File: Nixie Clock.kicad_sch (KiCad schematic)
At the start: 6 parts, among them J1 USB_C_Receptacle_USB2.0, U1 ESP32-S2-WROVER

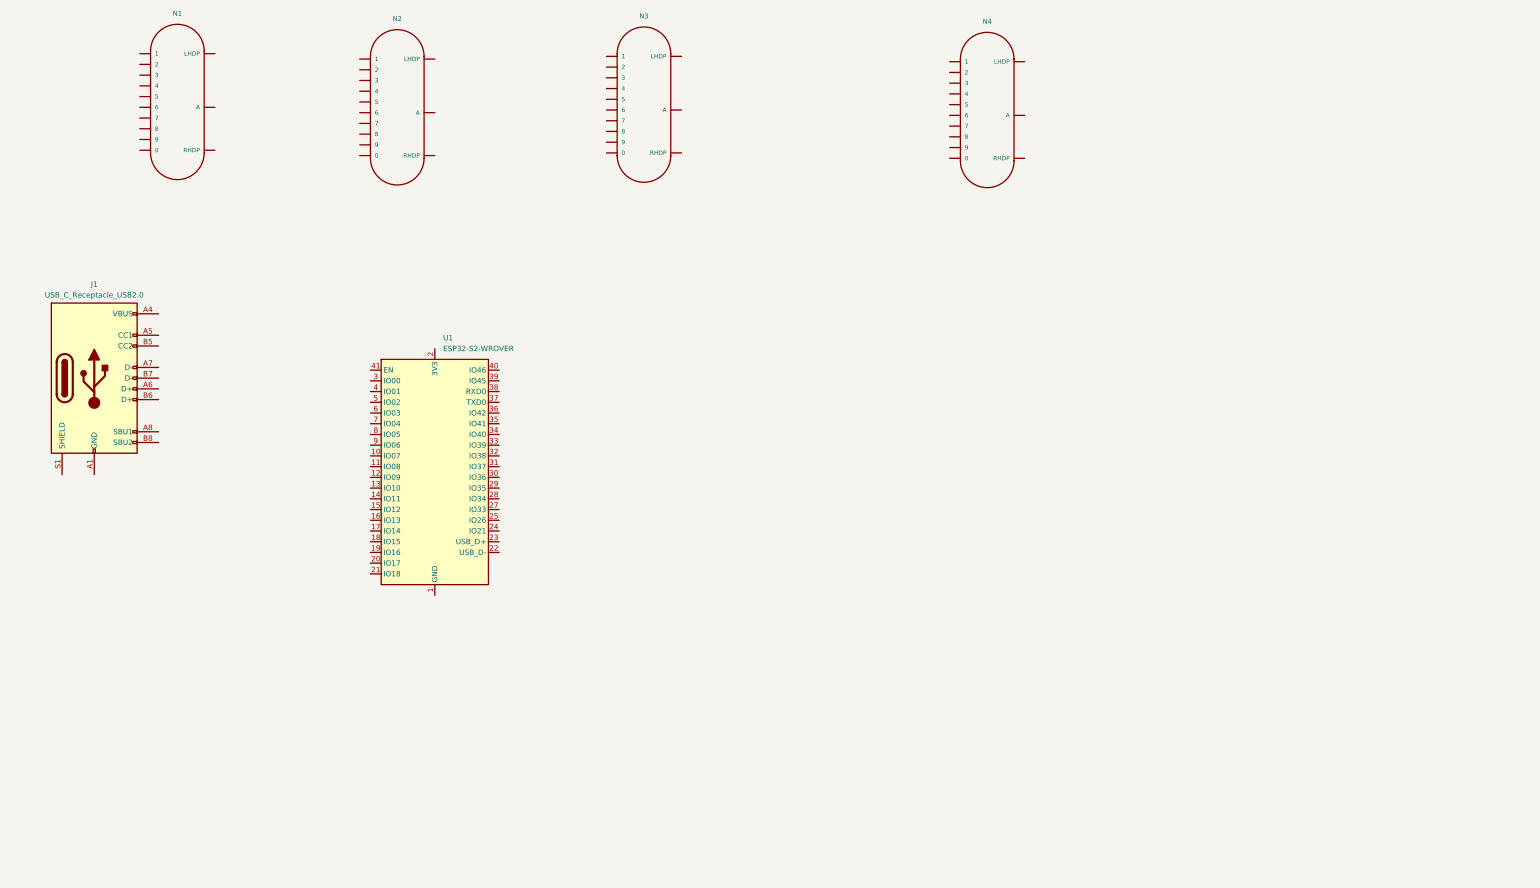
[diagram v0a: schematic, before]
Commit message: Finalized Bottom Plate with Gerbers
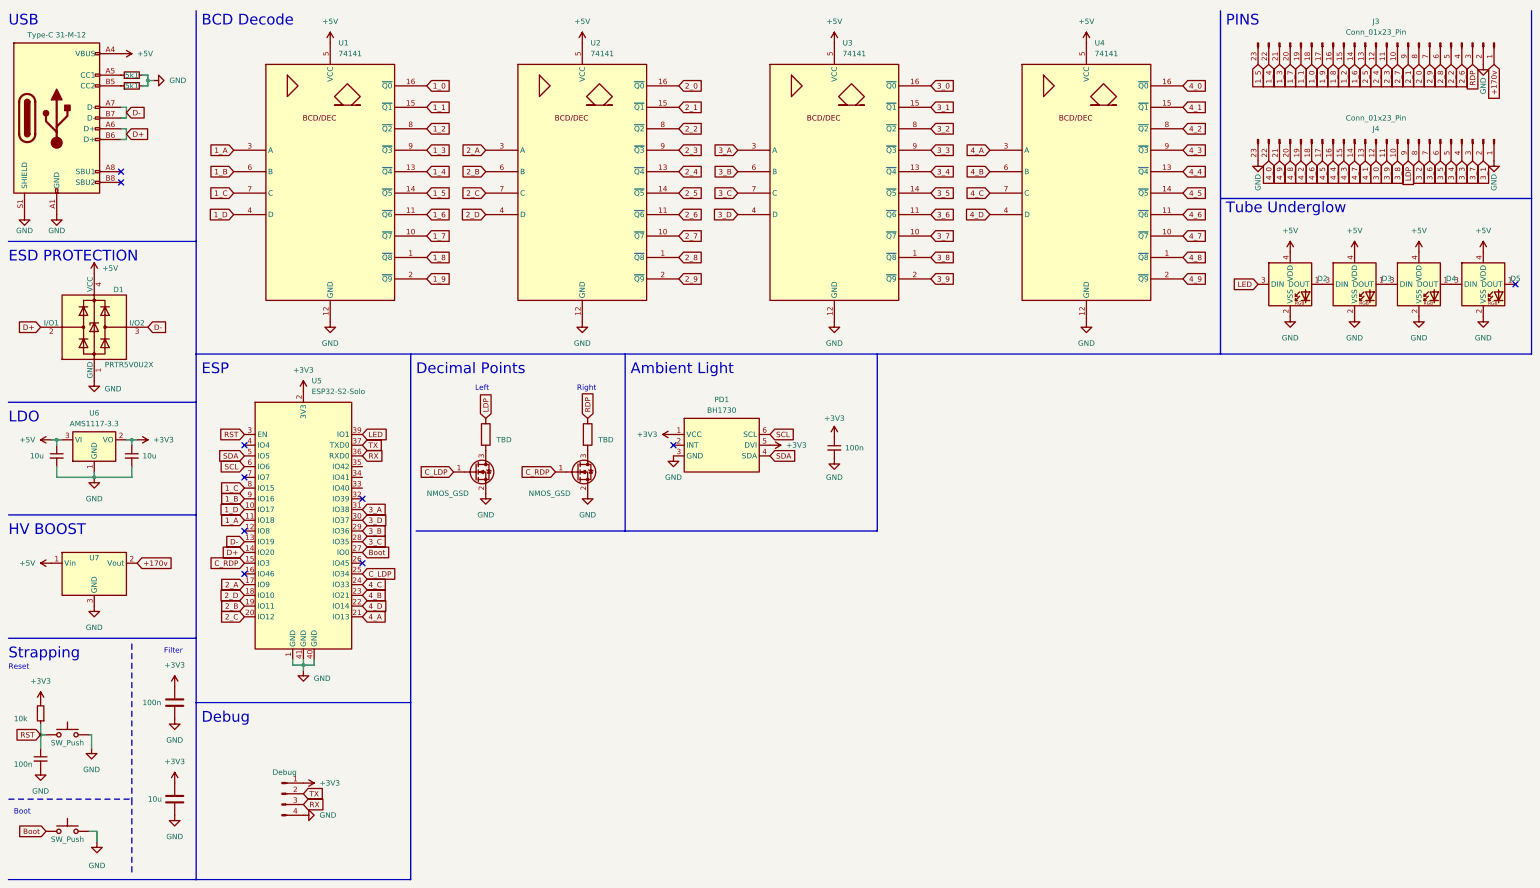
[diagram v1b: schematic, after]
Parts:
- removed N1, N2, N3, N4: IN-16, nixies-us:nixies-us-IN-16, symbol nixies-us:IN-16
- removed U1: ESP32-S2-WROVER, RF_Module:ESP32-S3-WROOM-1, symbol RF_Module:ESP32-S2-WROVER
- added C1, C2: 10u, Capacitor_SMD:C_0603_1608Metric, symbol Device:C_Small
- added C3: 10u, Capacitor_SMD:C_0603_1608Metric, symbol Device:C
- added C4: 100n, Capacitor_SMD:C_0402_1005Metric, symbol Device:C
- added C5, C6: 100n, Capacitor_SMD:C_0402_1005Metric, symbol Device:C_Small
- added D1: PRTR5V0U2X, Package_TO_SOT_SMD:SOT-143, symbol Power_Protection:PRTR5V0U2X
- added D2, D3, D4, D5: ~, LED_SMD:LED_WS2812B-2020_PLCC4_2.0x2.0mm, symbol WorldSemi_LED:WS2812B-2020
- added J2: Debug, Connector_PinHeader_2.54mm:PinHeader_1x04_P2.54mm_Vertical, symbol Connector:Conn_01x04_Pin
- added J3, J4: Conn_01x23_Pin, Connector_PinSocket_2.54mm:PinSocket_1x23_P2.54mm_Vertical, symbol Connector:Conn_01x23_Pin
- added PD1: BH1730, Sensor_Ambient:WSOF6, symbol BH1730:BH1730
- added Q1, Q2: NMOS_GSD, Package_TO_SOT_SMD:SOT-23, symbol Device:Q_NMOS_GSD
- added R1, R2: 5k1, Resistor_SMD:R_0402_1005Metric, symbol Device:R_Small
- added R3: 10k, Resistor_SMD:R_0402_1005Metric, symbol Device:R_Small
- added R4, R5: TBD, Resistor_SMD:R_0603_1608Metric_Pad0.98x0.95mm_HandSolder, symbol Device:R
- added RST1, SW2: SW_Push, Button_Switch_SMD:SW_SPST_SKQG_WithStem, symbol Switch:SW_Push
- added U1, U2, U3, U4: 74141, Package_DIP:DIP-16_W7.62mm, symbol 74xx_IEEE:74141
- added U5: ESP32-S2-Solo, RF_Module:ESP32-S3-WROOM-1, symbol ESP:ESP32-S2-Solo
- added U6: AMS1117-3.3, Package_TO_SOT_SMD:SOT-223-3_TabPin2, symbol Regulator_Linear:AMS1117-3.3
- added U7: ~, omnixie:8200HV, symbol omnixie:8200HV
- J1: value USB_C_Receptacle_USB2.0 -> Type-C 31-M-12
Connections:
- net GND: now reaches J1.A1 (GND), J1.A12 (GND), J1.B1 (GND), J1.B12 (GND)
- net GND: now also J1.S1 (SHIELD), C1.2, C2.2, C3.2, C4.2, C5.2, C6.2, D1.1 (GND), D2.2 (VSS), D3.2 (VSS), D4.2 (VSS), D5.2 (VSS), J2.4 (Pin_4), J3.2 (Pin_2), J4.1 (Pin_1), J4.23 (Pin_23), PD1.3 (GND), Q1.2 (S), Q2.2 (S), R1.2, R2.2, RST1.2, SW2.2, U1.12 (GND), U2.12 (GND), U3.12 (GND), U4.12 (GND), U5.1 (GND), U5.40 (GND), U5.41 (GND), U6.1 (GND), U7.3 (GND)
- net +5V: now reaches J1.A4 (VBUS), J1.A9 (VBUS), J1.B4 (VBUS), J1.B9 (VBUS)
- net +5V: now also C1.1, D1.4 (VCC), D2.4 (VDD), D3.4 (VDD), D4.4 (VDD), D5.4 (VDD), U1.5 (VCC), U2.5 (VCC), U3.5 (VCC), U4.5 (VCC), U6.3 (VI), U7.1 (Vin)
- net at J1.A5 (CC1): now also R1.1
- net D+: now reaches J1.A6 (D+)
- net D+: now also J1.B6 (D+), D1.2 (I/O1), U5.14 (IO20)
- net D-: now reaches J1.A7 (D-)
- net D-: now also J1.B7 (D-), D1.3 (I/O2), U5.13 (IO19)
- net at J1.B5 (CC2): now also R2.1
- new net: D4.1 (DOUT), D5.3 (DIN)
- new net: D3.1 (DOUT), D4.3 (DIN)
- new net: Q1.3 (D), R4.2
- new net: Q2.3 (D), R5.2
- new net: D2.1 (DOUT), D3.3 (DIN)
- new net +170v: J3.1 (Pin_1), U7.2 (Vout)
- new net +3V3: C2.1, C3.1, C4.1, C6.1, J2.1 (Pin_1), PD1.1 (VCC), PD1.5 (DVI), R3.2, U5.2 (3V3), U6.2 (VO)
- new net 1_0: J3.18 (Pin_18), U1.16 (~{Q0})
- new net 1_1: J3.19 (Pin_19), U1.15 (~{Q1})
- new net 1_2: J3.15 (Pin_15), U1.8 (~{Q2})
- new net 1_3: J3.21 (Pin_21), U1.9 (~{Q3})
- new net 1_4: J3.22 (Pin_22), U1.13 (~{Q4})
- new net 1_5: J3.23 (Pin_23), U1.14 (~{Q5})
- new net 1_6: J3.14 (Pin_14), U1.11 (~{Q6})
- new net 1_7: J3.20 (Pin_20), U1.10 (~{Q7})
- new net 1_8: J3.16 (Pin_16), U1.1 (~{Q8})
- new net 1_9: J3.17 (Pin_17), U1.2 (~{Q9})
- new net 1_A: U1.3 (A), U5.11 (IO18)
- new net 1_B: U1.6 (B), U5.9 (IO16)
- new net 1_C: U1.7 (C), U5.8 (IO15)
- new net 1_D: U1.4 (D), U5.10 (IO17)
- new net 2_0: J3.8 (Pin_8), U2.16 (~{Q0})
- new net 2_1: J3.9 (Pin_9), U2.15 (~{Q1})
- new net 2_2: J3.5 (Pin_5), U2.8 (~{Q2})
- new net 2_3: J3.11 (Pin_11), U2.9 (~{Q3})
- new net 2_4: J3.12 (Pin_12), U2.13 (~{Q4})
- new net 2_5: J3.13 (Pin_13), U2.14 (~{Q5})
- new net 2_6: J3.4 (Pin_4), U2.11 (~{Q6})
- new net 2_7: J3.10 (Pin_10), U2.10 (~{Q7})
- new net 2_8: J3.6 (Pin_6), U2.1 (~{Q8})
- new net 2_9: J3.7 (Pin_7), U2.2 (~{Q9})
- new net 2_A: U2.3 (A), U5.17 (IO9)
- new net 2_B: U2.6 (B), U5.19 (IO11)
- new net 2_C: U2.7 (C), U5.20 (IO12)
- new net 2_D: U2.4 (D), U5.18 (IO10)
- new net 3_0: J4.12 (Pin_12), U3.16 (~{Q0})
- new net 3_1: J4.2 (Pin_2), U3.15 (~{Q1})
- new net 3_2: J4.8 (Pin_8), U3.8 (~{Q2})
- new net 3_3: J4.4 (Pin_4), U3.9 (~{Q3})
- new net 3_4: J4.5 (Pin_5), U3.13 (~{Q4})
- new net 3_5: J4.6 (Pin_6), U3.14 (~{Q5})
- new net 3_6: J4.7 (Pin_7), U3.11 (~{Q6})
- new net 3_7: J4.3 (Pin_3), U3.10 (~{Q7})
- new net 3_8: J4.10 (Pin_10), U3.1 (~{Q8})
- new net 3_9: J4.11 (Pin_11), U3.2 (~{Q9})
- new net 3_A: U3.3 (A), U5.31 (IO38)
- new net 3_B: U3.6 (B), U5.29 (IO36)
- new net 3_C: U3.7 (C), U5.28 (IO35)
- new net 3_D: U3.4 (D), U5.30 (IO37)
- new net 4_0: J4.22 (Pin_22), U4.16 (~{Q0})
- new net 4_1: J4.13 (Pin_13), U4.15 (~{Q1})
- new net 4_2: J4.19 (Pin_19), U4.8 (~{Q2})
- new net 4_3: J4.15 (Pin_15), U4.9 (~{Q3})
- new net 4_4: J4.16 (Pin_16), U4.13 (~{Q4})
- new net 4_5: J4.17 (Pin_17), U4.14 (~{Q5})
- new net 4_6: J4.18 (Pin_18), U4.11 (~{Q6})
- new net 4_7: J4.14 (Pin_14), U4.10 (~{Q7})
- new net 4_8: J4.20 (Pin_20), U4.1 (~{Q8})
- new net 4_9: J4.21 (Pin_21), U4.2 (~{Q9})
- new net 4_A: U4.3 (A), U5.21 (IO13)
- new net 4_B: U4.6 (B), U5.23 (IO21)
- new net 4_C: U4.7 (C), U5.24 (IO33)
- new net 4_D: U4.4 (D), U5.22 (IO14)
- new net Boot: SW2.1, U5.27 (IO0)
- new net C_LDP: Q2.1 (G), U5.25 (IO34)
- new net C_RDP: Q1.1 (G), U5.15 (IO3)
- new net LDP: J4.9 (Pin_9), R5.1
- new net LED: D2.3 (DIN), U5.39 (IO1)
- new net RDP: J3.3 (Pin_3), R4.1
- new net RST: C5.1, R3.1, RST1.1, U5.3 (EN)
- new net RX: J2.3 (Pin_3), U5.36 (RXD0)
- new net SCL: PD1.6 (SCL), U5.6 (IO6)
- new net SDA: PD1.4 (SDA), U5.5 (IO5)
- new net TX: J2.2 (Pin_2), U5.37 (TXD0)
- no-connect marks 0 -> 10
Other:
- note added: "Ambient Light"
- note added: "BCD Decode"
- note added: "Boot"
- note added: "Debug"
- note added: "Decimal Points"
- note added: "ESD PROTECTION"
- note added: "ESP"
- note added: "Filter"
- note added: "HV BOOST"
- note added: "LDO"
- note added: "Left"
- note added: "PINS"
- note added: "Reset"
- note added: "Right"
- note added: "Strapping"
- note added: "Tube Underglow"
- note added: "USB"
